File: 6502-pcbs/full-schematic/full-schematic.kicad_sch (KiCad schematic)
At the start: 62 parts, among them J1 Halt CLK, J2 1MHz CLK, J3 Barrel_Jack, SW1 Push, SW2 Push, SW3 SW_SPDT, U1 W65C02SxP, U10 74LS08, U11 74LS04, U12 74LS32, U13 ATmega644-20P, U14 74HC00, U15 74HC00, U16 74HC00, U2 HM62256BLP, U3 28C256, U4 W65C22SxP, U5 RC1602A, U6 W65C51NxP, U7 NE555P, U8 NE555P, U9 NE555P, Y1 ACO-xxxMHz

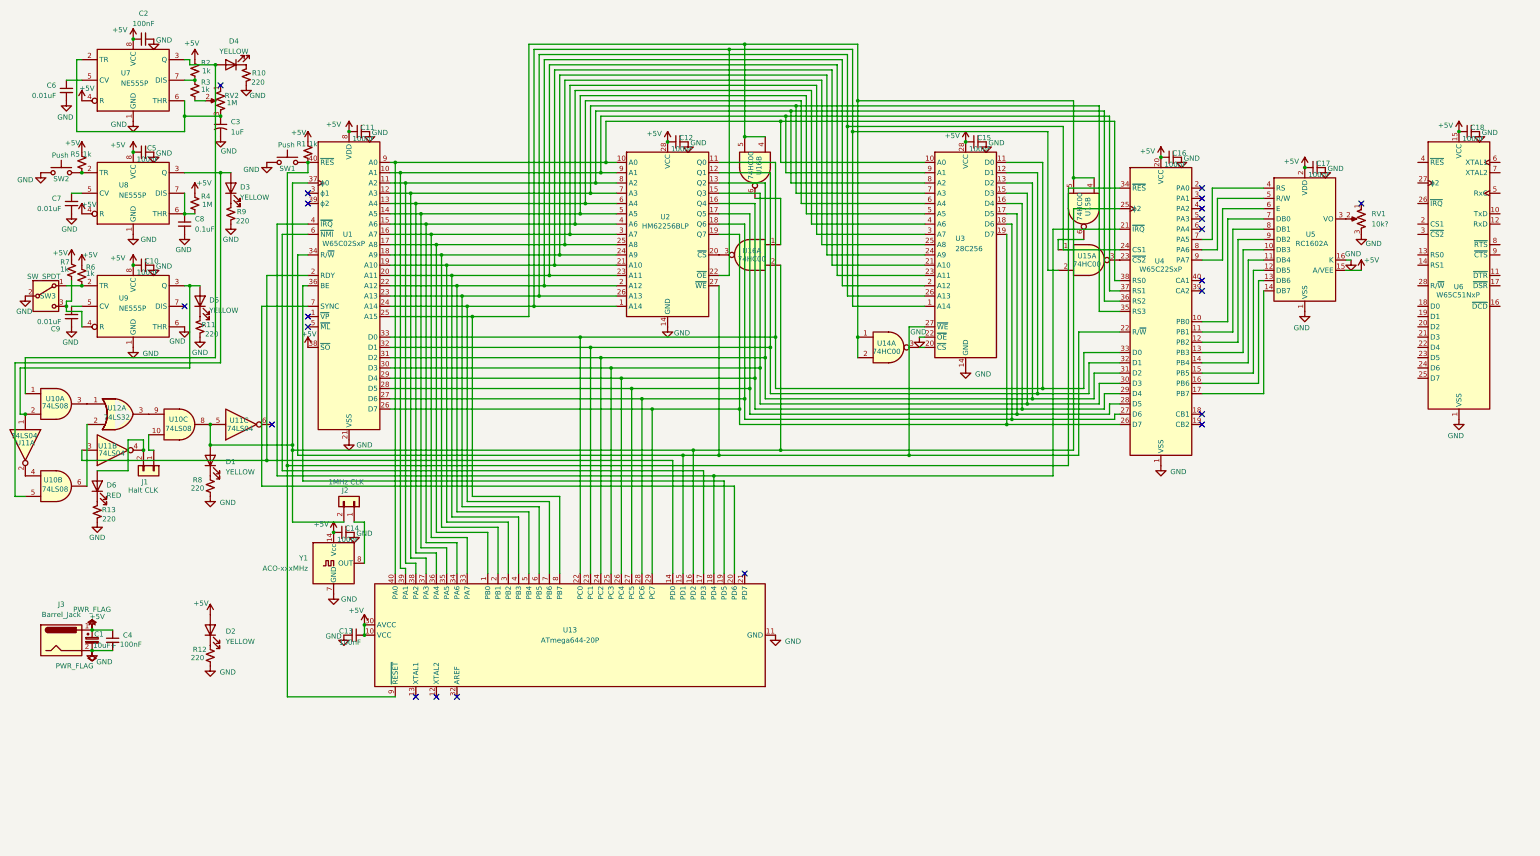
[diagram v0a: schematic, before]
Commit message: 28c256 rom
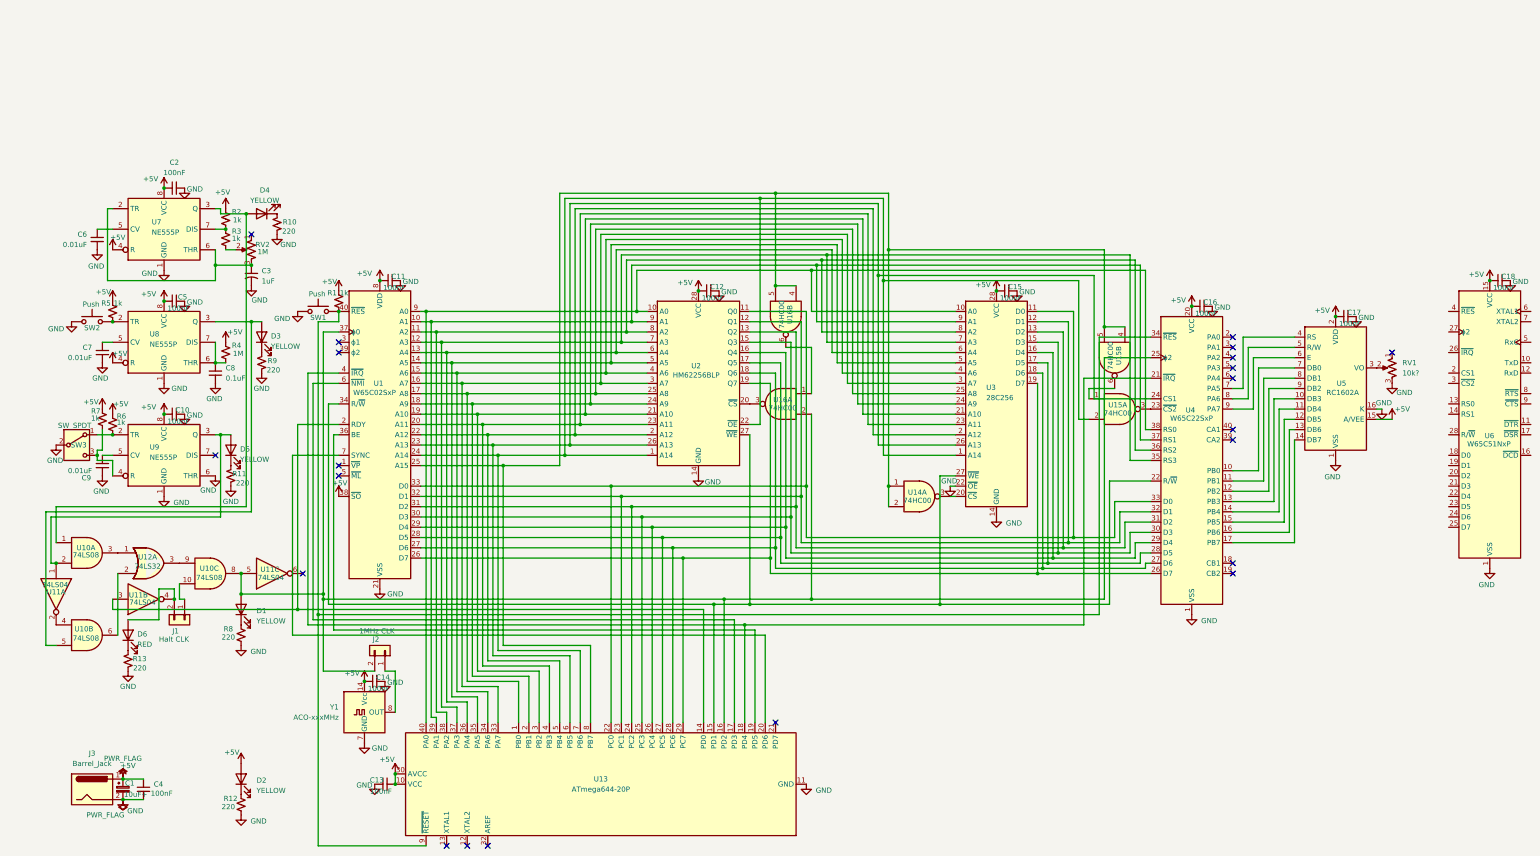
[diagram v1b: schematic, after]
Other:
- company: (none) -> Sam Warr
- title: (none) -> 6502 Stacked
- moved on the sheet: C1, C10, C11, C12, C13, C14, C15, C16, C17, C18, C2, C3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
